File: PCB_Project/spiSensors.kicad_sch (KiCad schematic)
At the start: 10 parts

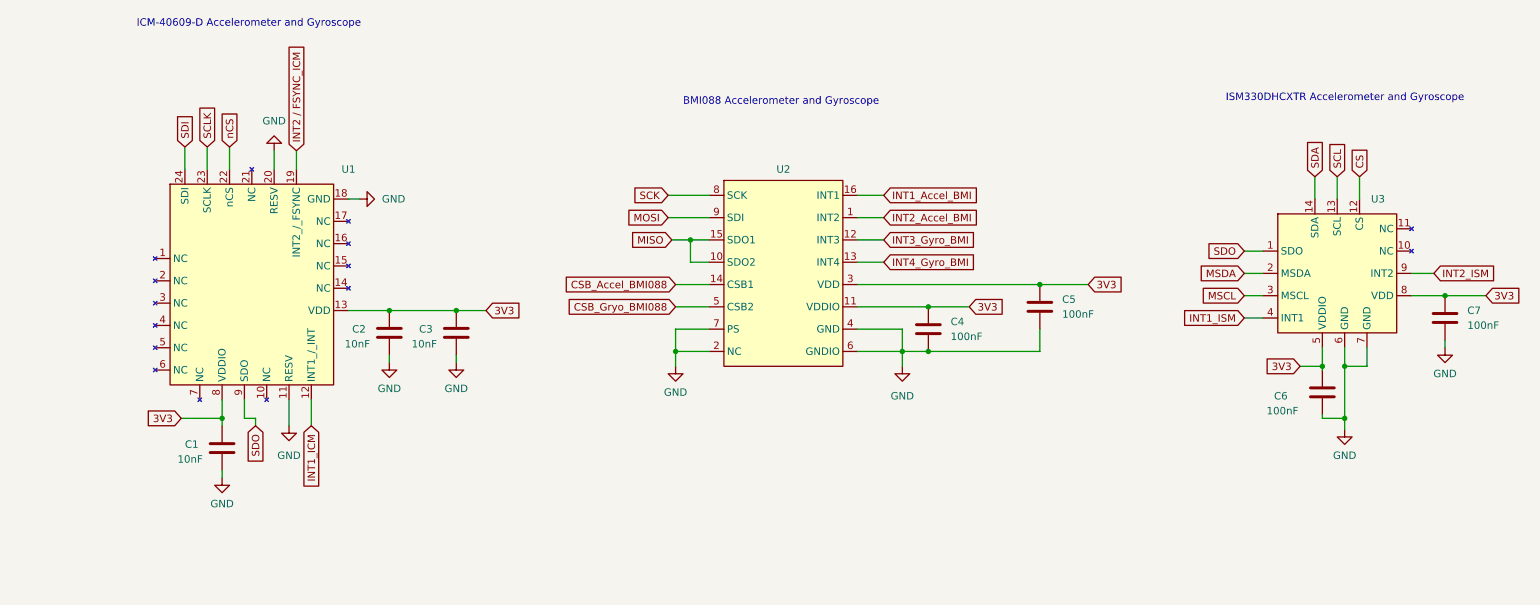
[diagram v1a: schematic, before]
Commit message: work baby
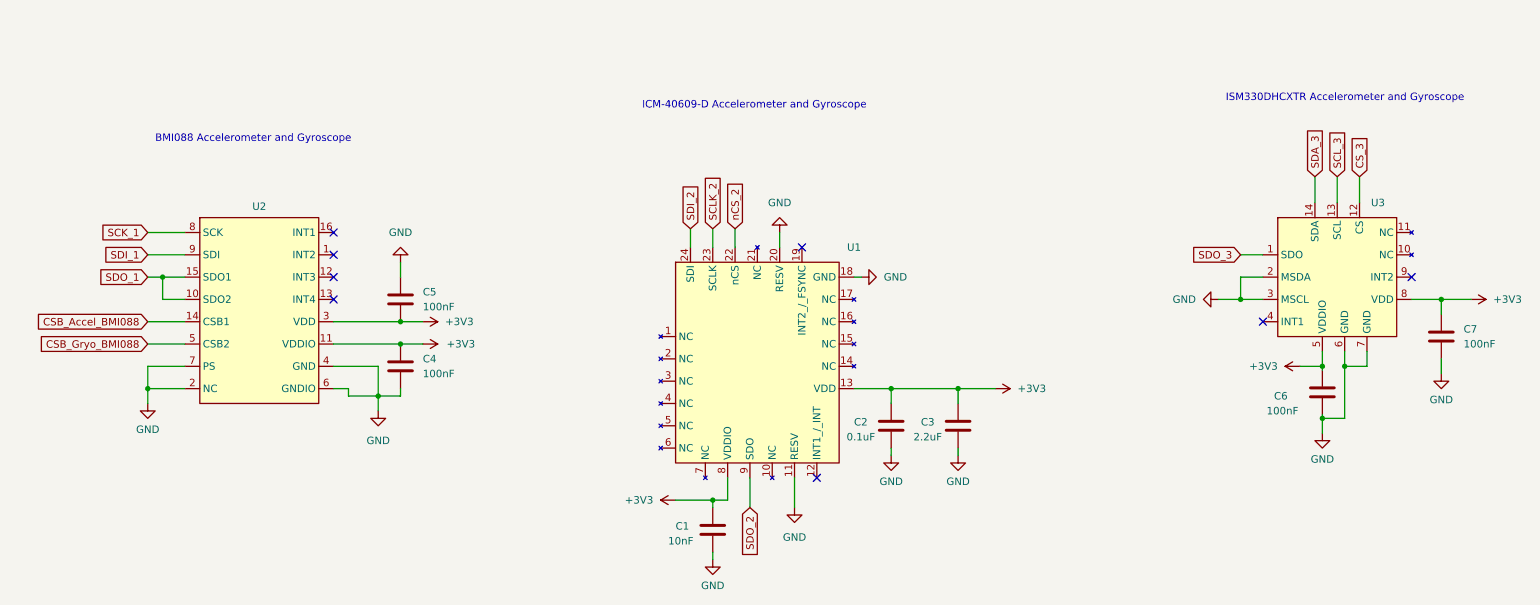
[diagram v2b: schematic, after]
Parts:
- C1, C4, C5, C6, C7: footprint (none) -> Capacitor_SMD:C_0603_1608Metric
- C2: value 10nF -> 0.1uF; footprint (none) -> Capacitor_SMD:C_0402_1005Metric
- C3: value 10nF -> 2.2uF; footprint (none) -> Capacitor_SMD:C_0402_1005Metric
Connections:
- net MSCL is gone; now on net GND: U3.3 (MSCL)
- net MSDA is gone; now on net GND: U3.2 (MSDA)
- net 3V3 renamed +3V3
- net CS renamed CS_3
- net INT1_Accel_BMI: no longer names the net of U2.16 (INT1)
- net INT1_ICM: no longer names the net of U1.12 (INT1_/_INT)
- net INT1_ISM: no longer names the net of U3.4 (INT1)
- net INT2 / FSYNC_ICM: no longer names the net of U1.19 (INT2_/_FSYNC)
- net INT2_Accel_BMI: no longer names the net of U2.1 (INT2)
- net INT2_ISM: no longer names the net of U3.9 (INT2)
- net INT3_Gyro_BMI: no longer names the net of U2.12 (INT3)
- net INT4_Gyro_BMI: no longer names the net of U2.13 (INT4)
- net MISO renamed SDO_1
- net MOSI renamed SDI_1
- net SCK renamed SCK_1
- net SCL renamed SCL_3
- net SCLK renamed SCLK_2
- net SDA renamed SDA_3
- net SDI renamed SDI_2
- net SDO renamed SDO_2
- net SDO_2: no longer U3.1 (SDO)
- net nCS renamed nCS_2
- new net SDO_3: U3.1 (SDO)
- no-connect marks 0 -> 8
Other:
- moved on the sheet: C1, C2, C3, C4, C5, C7, U1, U2, U3
